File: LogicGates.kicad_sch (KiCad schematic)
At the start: 48 parts, among them Q1 2N3904, Q10 2N3904, Q11 2N3904, Q12 2N3904, Q13 2N3904, Q14 2N3904, Q15 2N3904, Q16 2N3904, Q2 2N3904, Q3 2N3904, Q4 2N3904, Q5 2N3904, Q6 2N3904, Q7 2N3904, Q8 2N3904, Q9 2N3904, SW1 SW_DIP_x02

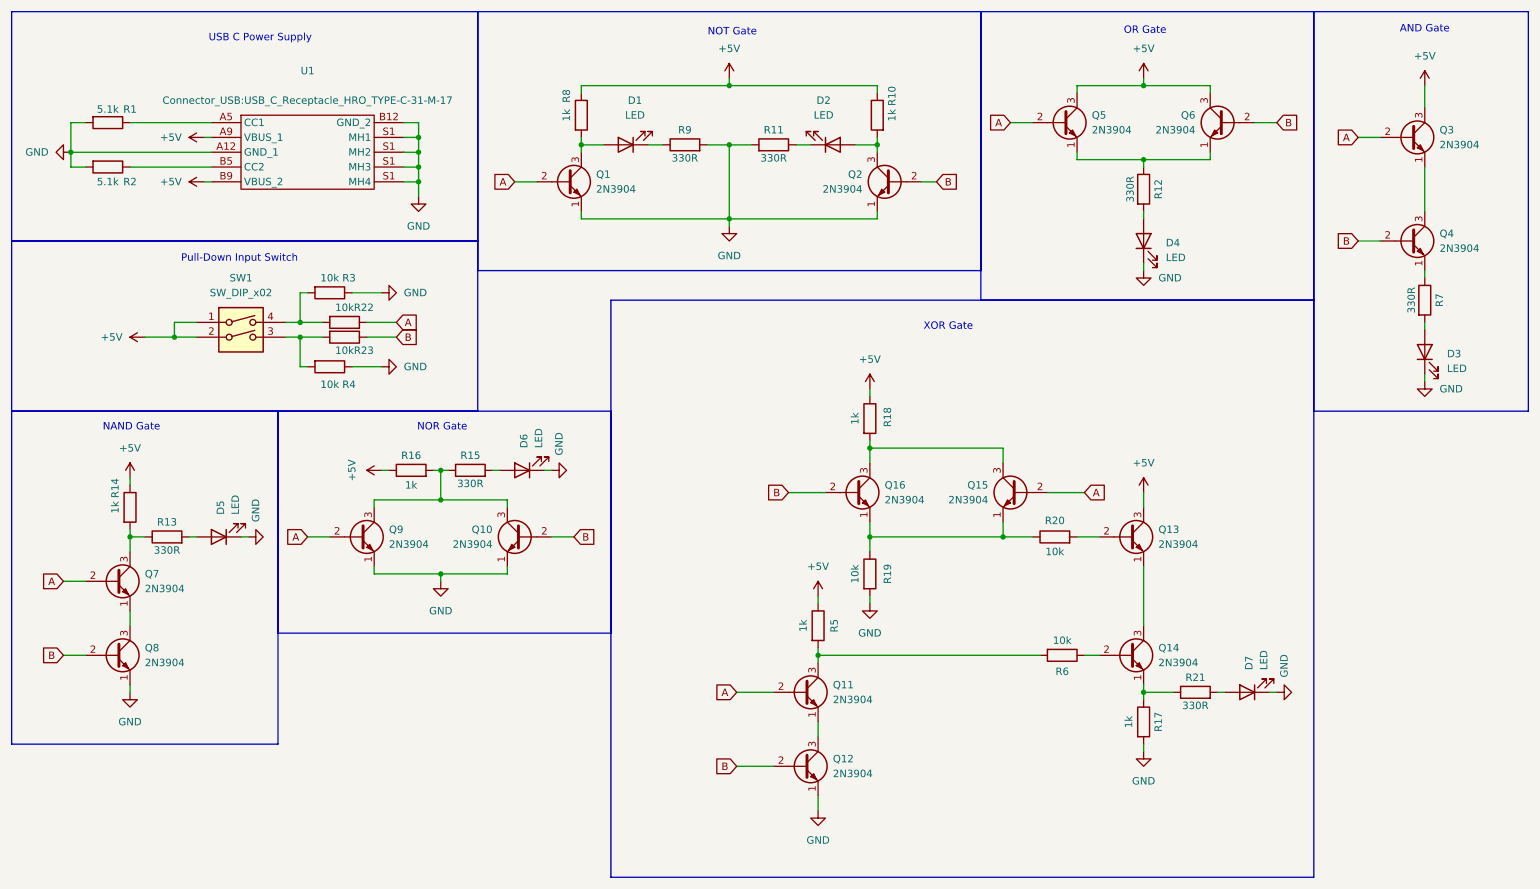
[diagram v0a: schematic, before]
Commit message: Add files via upload
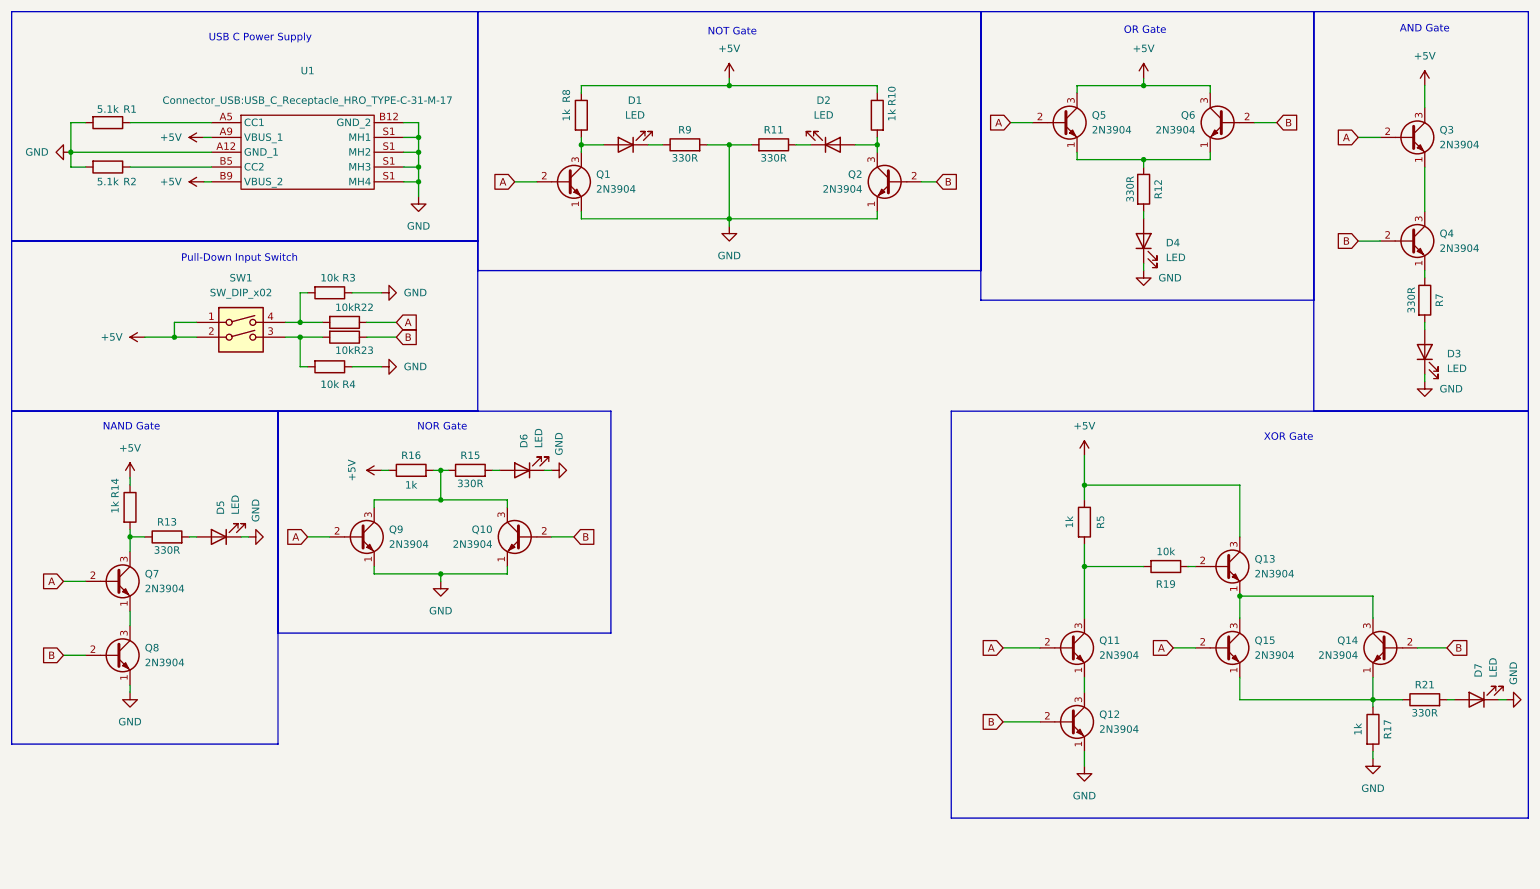
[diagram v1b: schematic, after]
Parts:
- removed Q16: 2N3904, Package_TO_SOT_THT:TO-92_Inline, symbol Transistor_BJT:2N3904
- removed R18: 1k, Resistor_SMD:R_0402_1005Metric, symbol Device:R
- removed R20, R6: 10k, Resistor_SMD:R_0402_1005Metric, symbol Device:R
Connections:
- net B: now also Q14.2 (B)
- net GND: no longer R19.2
- net at Q15.1 (E): now also Q14.1 (E), R17.1, R21.1; no longer R19.1
- net at Q15.3 (C): now also Q13.1 (E), Q14.3 (C)
- net at Q13.2 (B): now also R19.1
- net at Q11.3 (C), R5.2: now also R19.2
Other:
- moved on the sheet: D7, Q11, Q12, Q13, Q14, Q15, R17, R19, R21, R5
